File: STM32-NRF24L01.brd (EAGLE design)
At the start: 49.5 x 23 mm, 21 parts, among them IC1 STM32F030K6T6, IC2 MCP73811/2, IC3 SPX3819M5_3_3, J1 61301411121, J2 61301411121, P1 PUSH-SMD

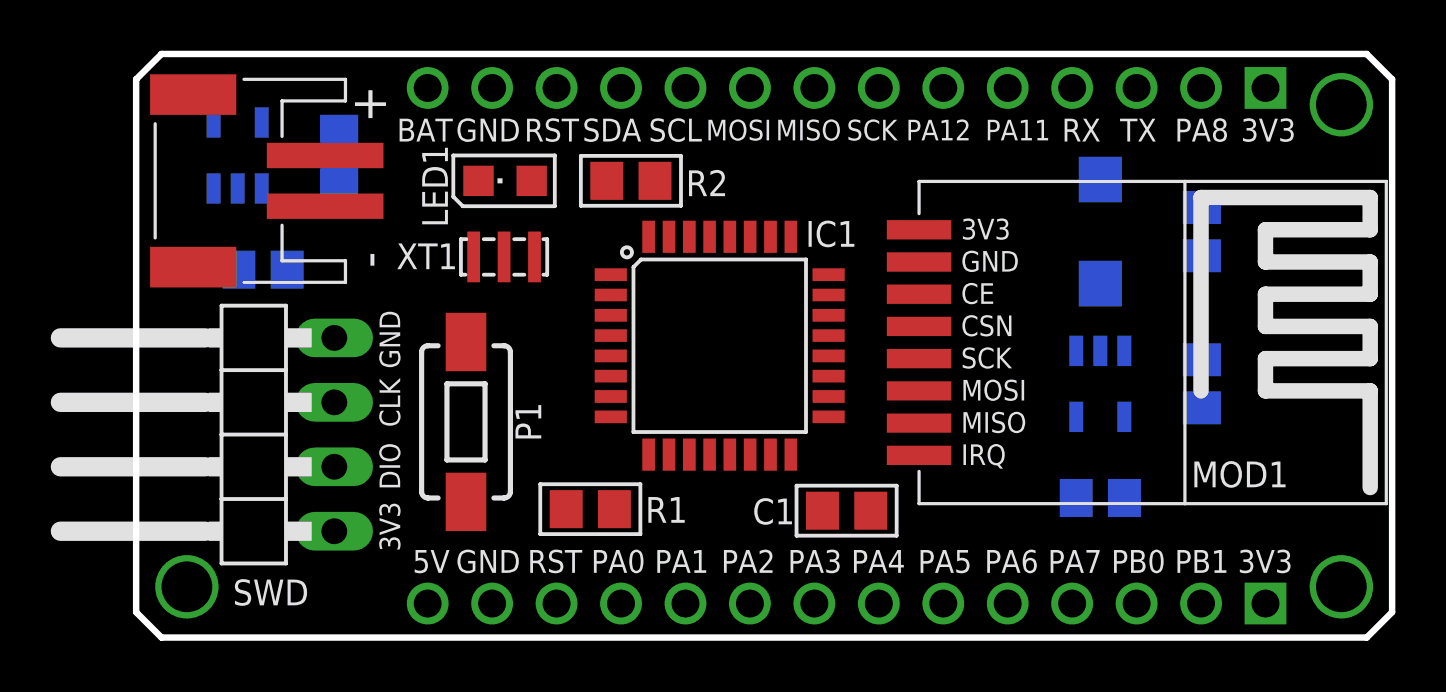
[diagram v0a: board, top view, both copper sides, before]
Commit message: Ruteo al 50%
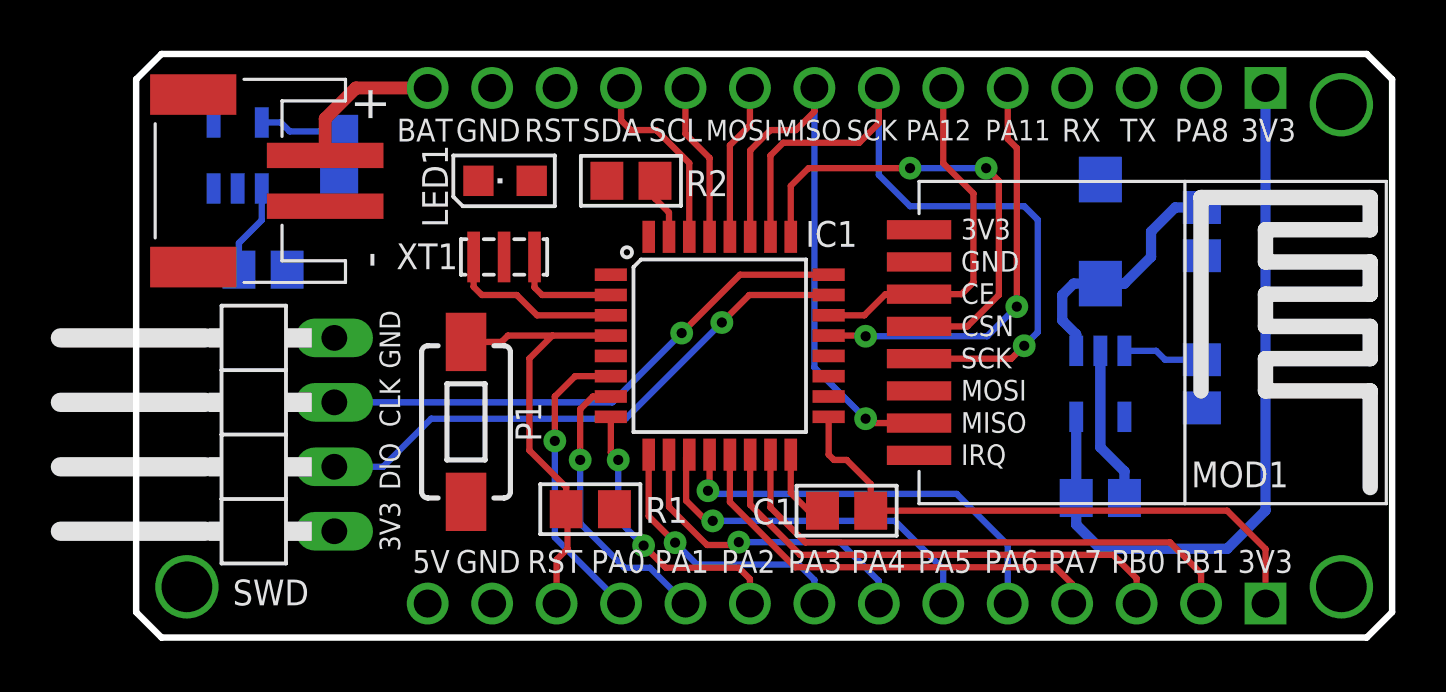
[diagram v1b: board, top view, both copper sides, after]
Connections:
- removed net PA11: IC1.21, J2.5
- removed net PA12: IC1.22, J2.6
- removed net PA8: IC1.18, J2.2
- net CE: now also IC1.22, J2.6
- net CSN: now also IC1.21, J2.5; no longer MOD1.5
- net IRQ: now also IC1.18, J2.2
- net NSS: now also MOD1.5
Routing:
- net +3V3: track 0.00 -> 52.4 mm
- net SCK: track 0.00 -> 29.4 mm, vias 0 -> 1
- net MISO: track 0.00 -> 23.6 mm, vias 0 -> 1
- net SWDIO: track 0.00 -> 22.3 mm, vias 0 -> 1
- net SWCLK: track 0.00 -> 21.6 mm, vias 0 -> 1
- net PB1: track 0.00 -> 21.3 mm
- net PB0: track 0.00 -> 19.4 mm
- net NSS: track 0.00 -> 18.9 mm, vias 0 -> 2
- net RST: track 0.00 -> 17.5 mm
- net AN7: track 0.00 -> 17.5 mm
- net CSN: track 0.00 -> 16.7 mm, vias 0 -> 2
- net AN6: track 0.00 -> 16.5 mm, vias 0 -> 1
- net CE: track 0.00 -> 14.4 mm
- net AN5: track 0.00 -> 14.3 mm, vias 0 -> 1
- net AN4: track 0.00 -> 12.5 mm, vias 0 -> 1
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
